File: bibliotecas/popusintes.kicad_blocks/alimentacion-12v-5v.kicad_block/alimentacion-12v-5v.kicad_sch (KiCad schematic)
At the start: 4 parts, among them J1 Conn_02x05_Odd_Even, U1 TL074

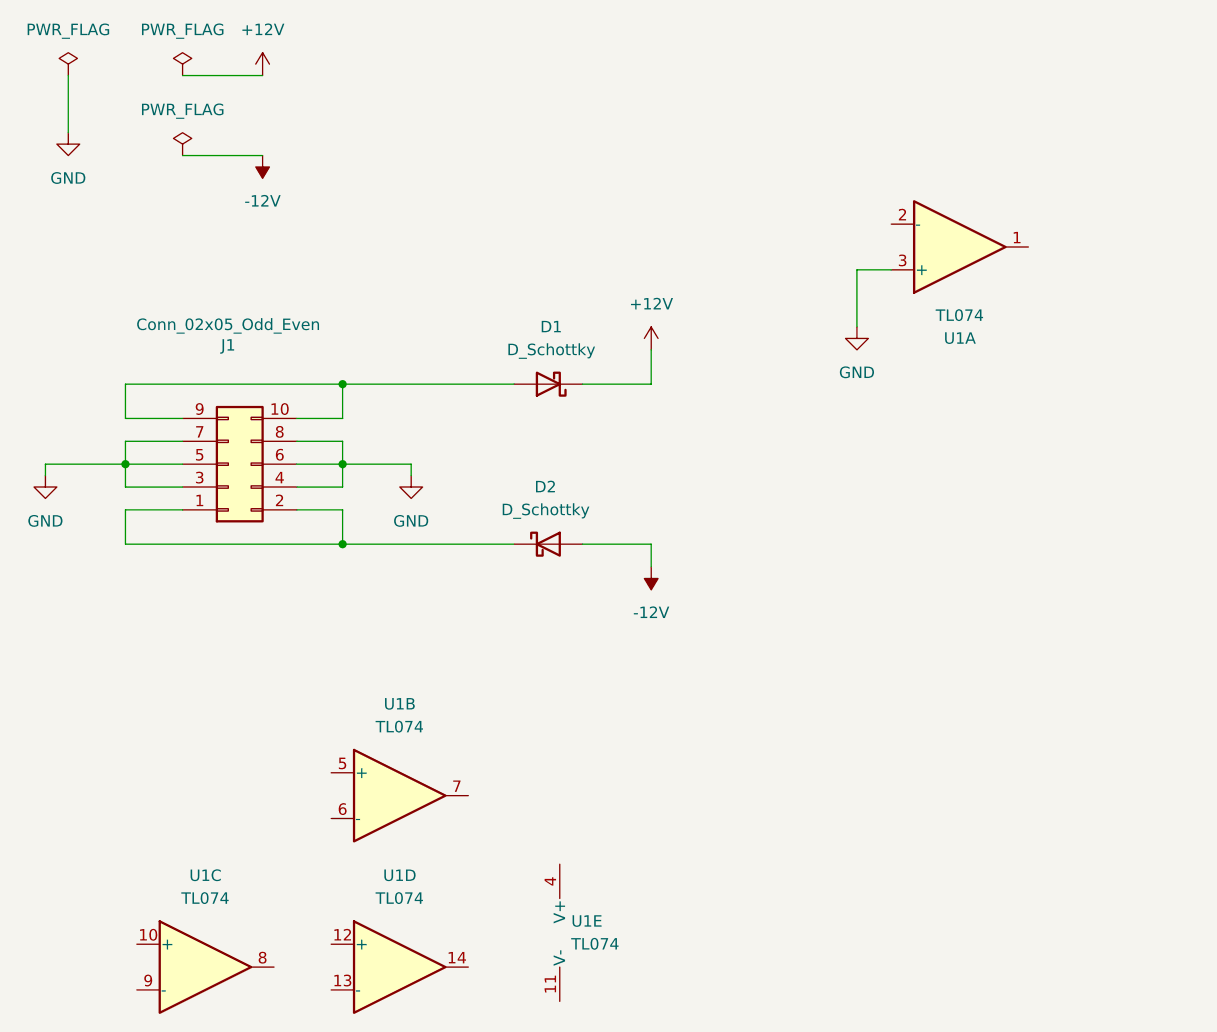
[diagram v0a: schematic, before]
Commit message: avanzar en lcsc, huellas, stock
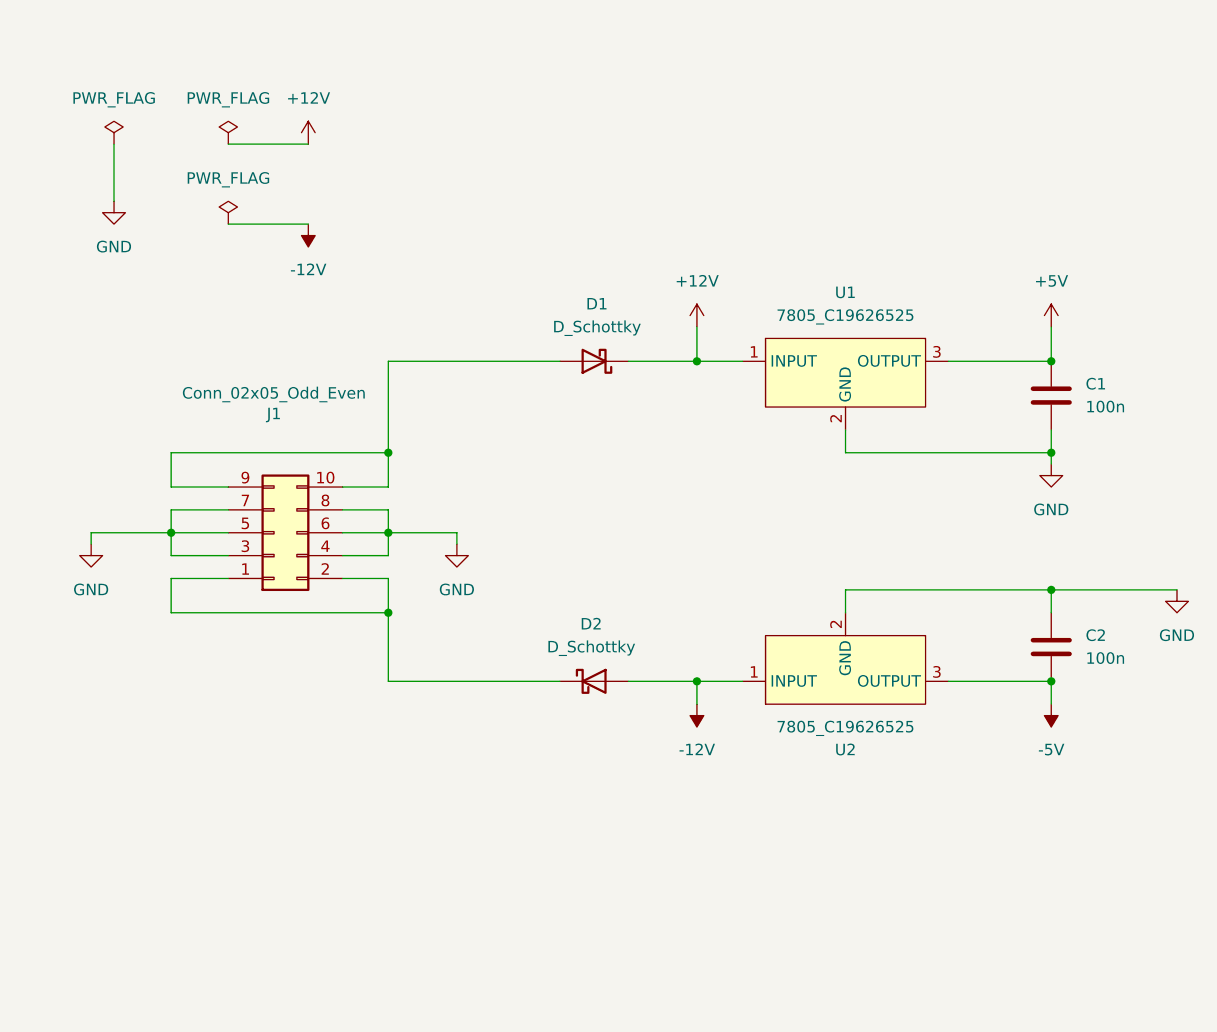
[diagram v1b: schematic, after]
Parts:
- removed U1: TL074, symbol Amplifier_Operational:TL074
- added C1, C2: 100n, Capacitor_SMD:C_0805_2012Metric_Pad1.18x1.45mm_HandSolder, symbol Device:C
- added U1, U2: 7805_C19626525, easyeda2kicad:TO-252-2_L6.6-W6.1-P4.57-LS9.9-BR-CW, symbol easyeda2kicad:7805_C19626525
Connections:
- net +12V: now also U1.1 (INPUT)
- net -12V: now also U2.1 (INPUT)
- net GND: now also C1.2, C2.1, U1.2 (GND), U2.2 (GND)
- new net +5V: C1.1, U1.3 (OUTPUT)
- new net -5V: C2.2, U2.3 (OUTPUT)
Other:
- title: (none) -> alimentacion-12v-5v
- moved on the sheet: D1, D2, J1
